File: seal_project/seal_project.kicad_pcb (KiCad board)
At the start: 2 copper layers, 72.2 x 63.6 mm, 6 parts, among them SW1 SW_SPDT

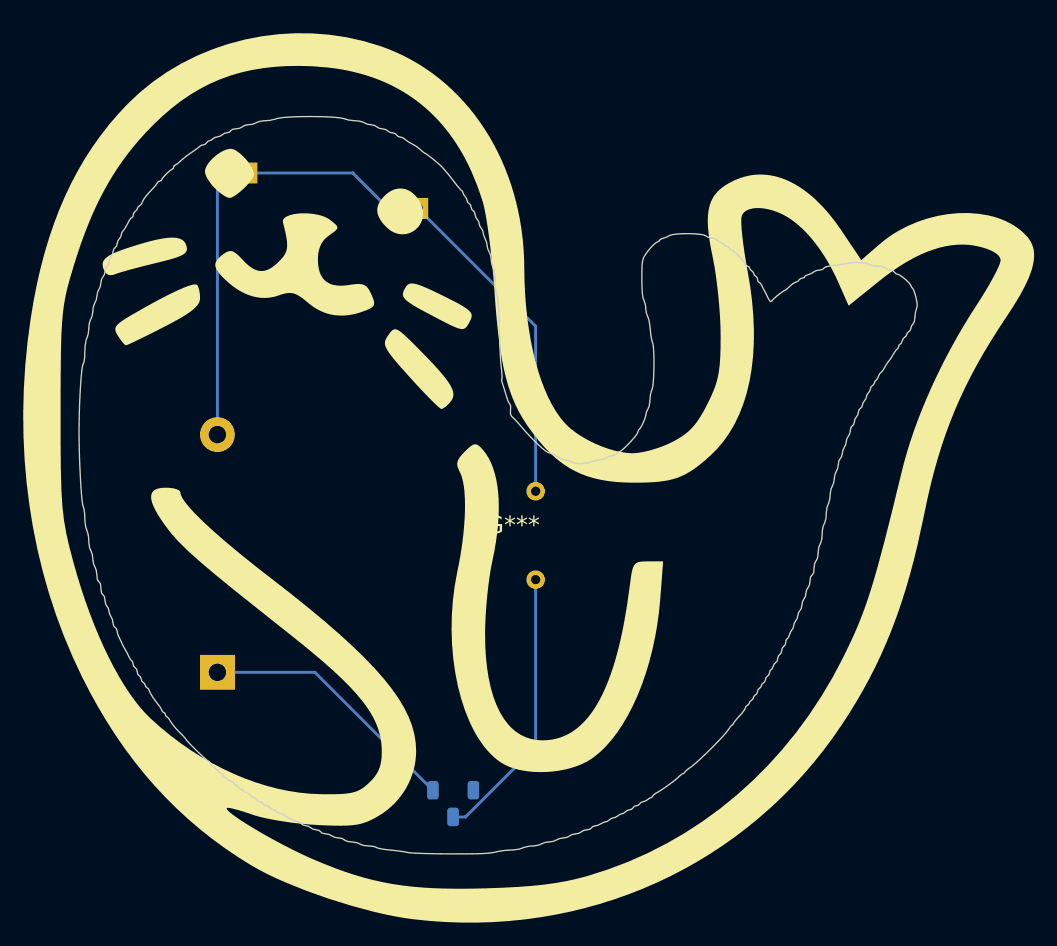
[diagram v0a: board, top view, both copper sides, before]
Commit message: final revisions
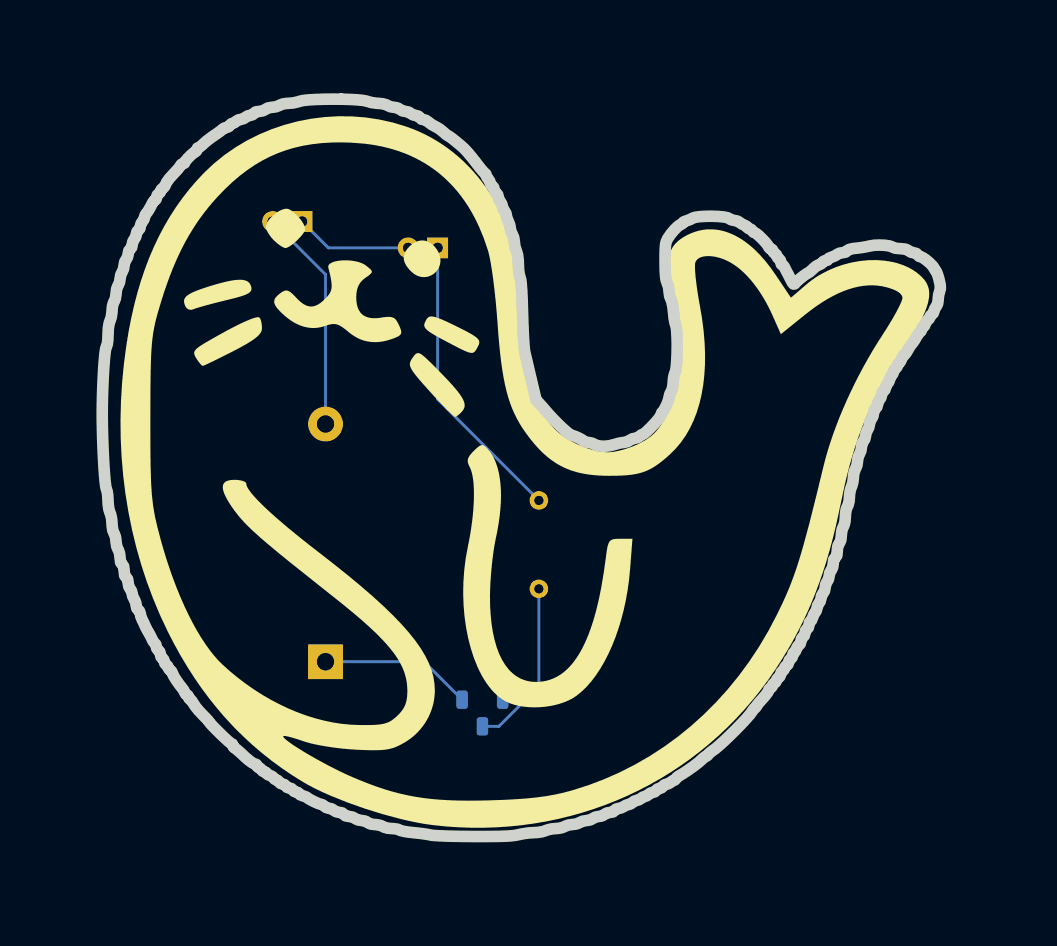
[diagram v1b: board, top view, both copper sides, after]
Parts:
- moved BT1 9.36 mm to (139.4, 115.3)
- moved SW1 8.20 mm to (152.9, 119.7)
- moved D1 6.34 mm to (137.3, 77.3)
- moved D2 3.81 mm to (149.0, 79.6)
- moved G*** 2.50 mm to (157.5, 102.0)
- moved R1 0.84 mm to (157.8, 109.0)
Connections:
- D1 pad 1: Net-(D1-K) -> Net-(BT1--)
- D1 pad 2: Net-(BT1--) -> Net-(D1-A)
- D2 pad 1: Net-(D2-K) -> Net-(D1-A)
- D2 pad 2: Net-(D1-K) -> Net-(D2-A)
- R1 pad 2: Net-(D2-K) -> Net-(D2-A)
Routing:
- net Net-(D2-K): track 28.6 -> 0.00 mm
- net (no net): track 0.00 -> 25.4 mm
- net Net-(D1-K): track 13.5 -> 0.00 mm
- net Net-(BT1-+): track 22.8 -> 13.1 mm
- net Net-(SW1-B): track 24.0 -> 14.7 mm
- net Net-(BT1--): track 22.5 -> 29.5 mm
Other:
- outline, holes or cut-outs redrawn

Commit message: updates, still debugging
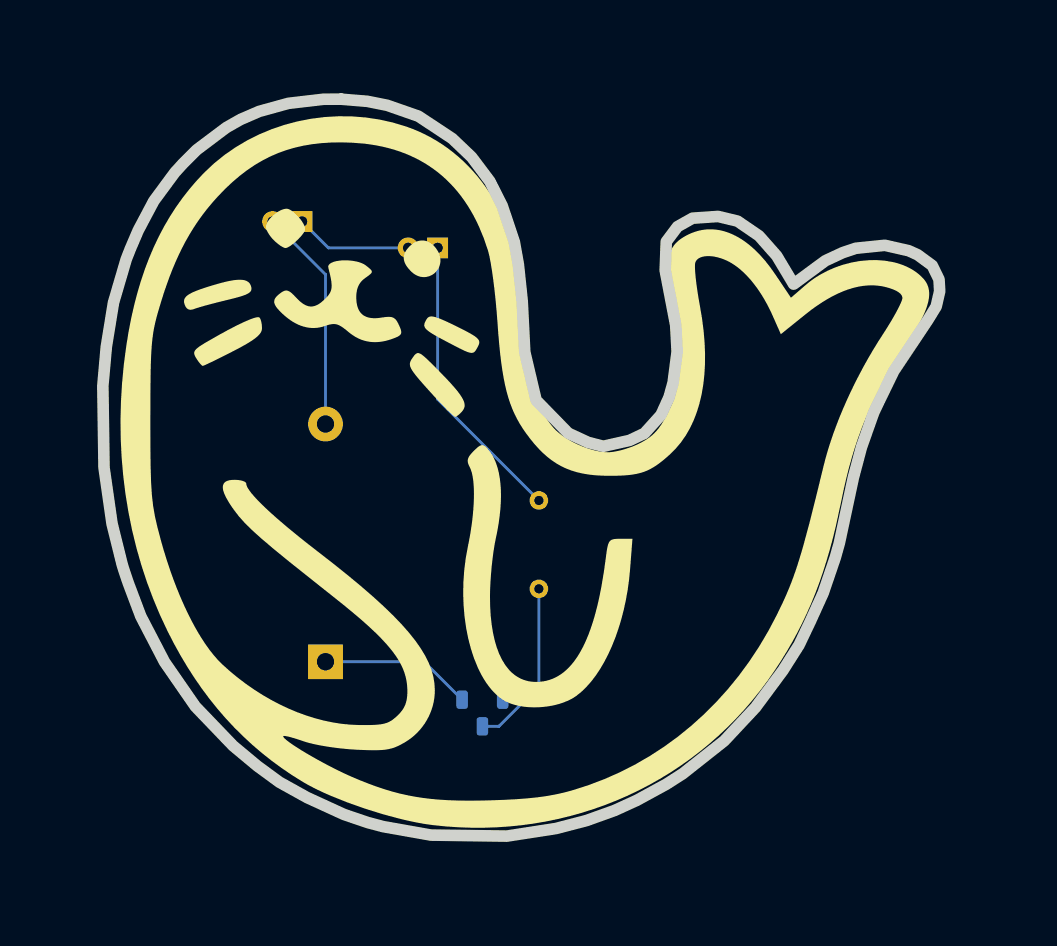
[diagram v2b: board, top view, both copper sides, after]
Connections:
- SW1 pad 3: unconnected-(SW1-C-Pad3) -> GND
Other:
- board size 72.2 x 63.6 mm -> 72.1 x 63.5 mm

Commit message: still buggy
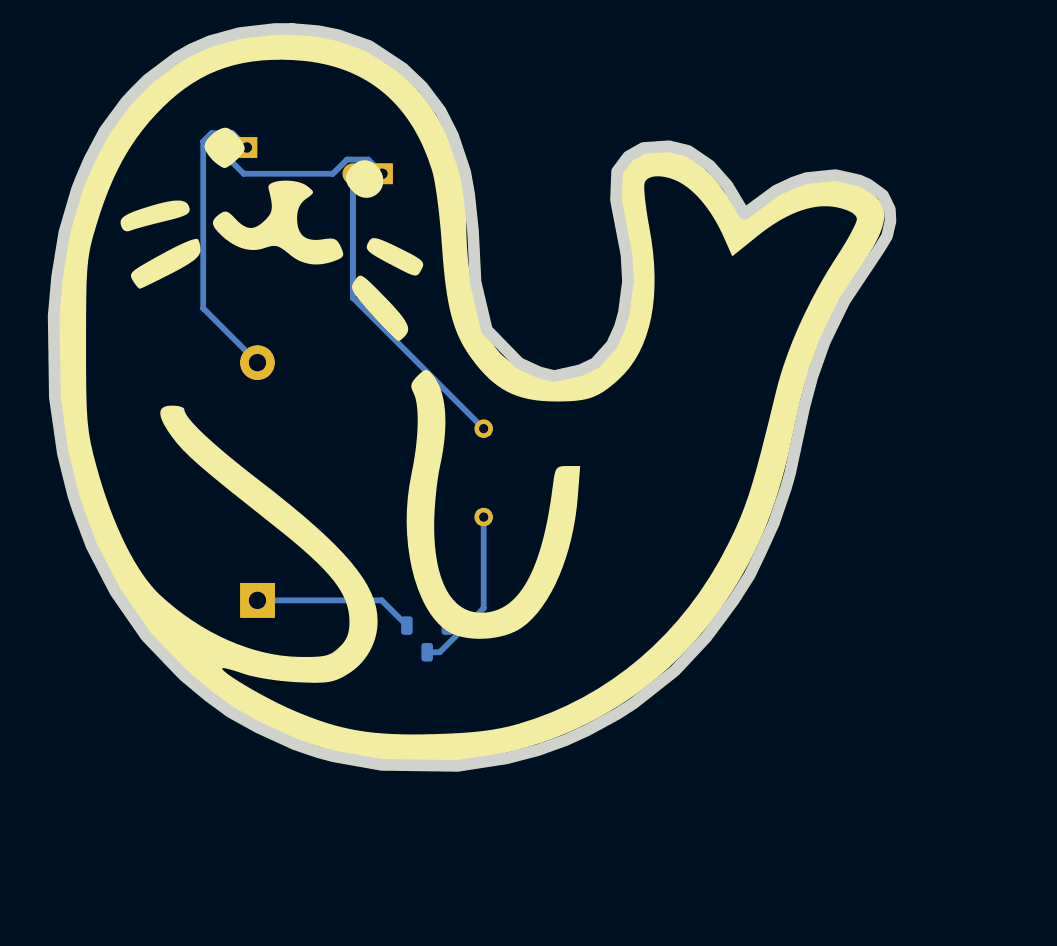
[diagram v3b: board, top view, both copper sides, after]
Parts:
- moved D1 7.96 mm to (132.6, 71.0)
- moved D2 7.96 mm to (144.3, 73.2)
- moved SW1 7.96 mm to (148.1, 113.3)
- moved BT1 7.90 mm to (133.5, 110.0)
- moved R1 7.81 mm to (153.0, 102.8)
- moved G*** 7.39 mm to (153.3, 95.9)
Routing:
- net Net-(D2-A): track 0.00 -> 26.6 mm
- net (no net): track 25.4 -> 0.00 mm
- net Net-(D1-A): track 0.00 -> 16.2 mm
- net Net-(BT1--): track 29.5 -> 25.6 mm
- net Net-(BT1-+): track 13.1 -> 13.8 mm
